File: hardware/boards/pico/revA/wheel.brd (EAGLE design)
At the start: 38 x 38 mm, 0 parts

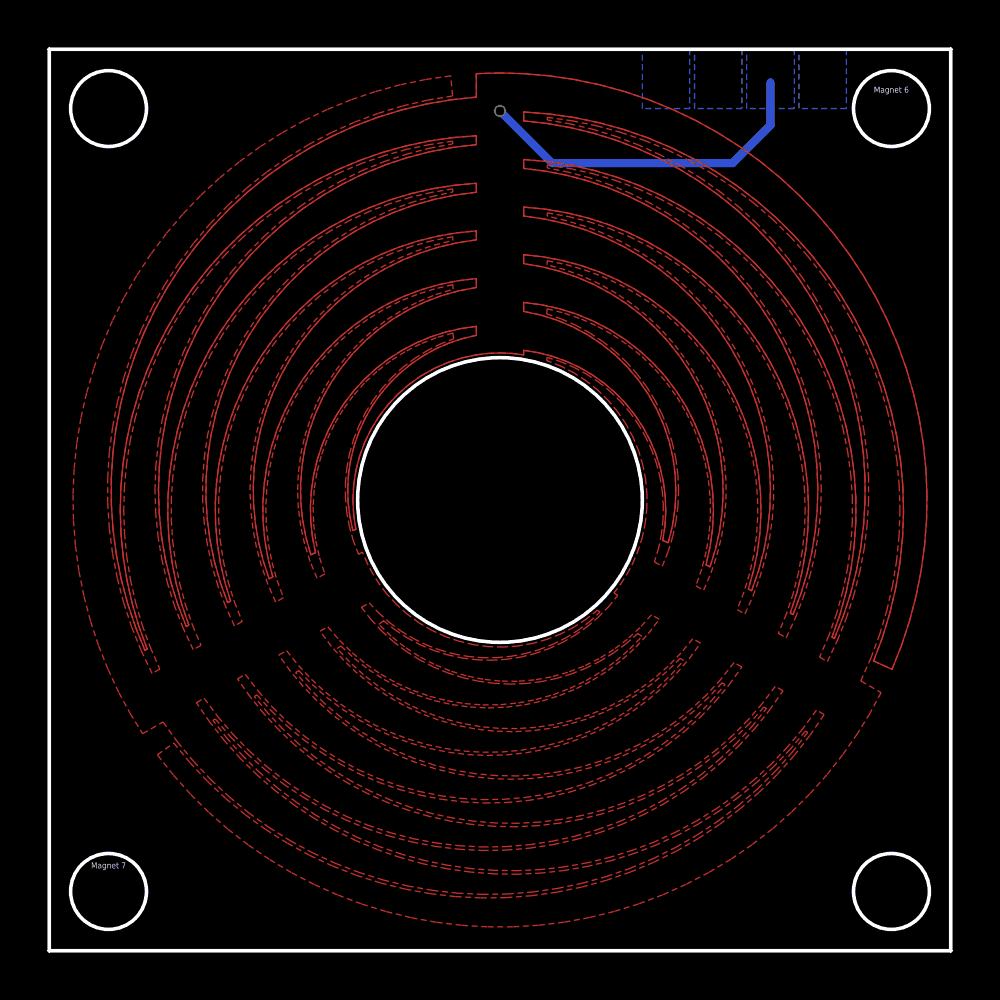
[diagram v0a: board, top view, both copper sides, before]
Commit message: pico: wheel board, basically complete
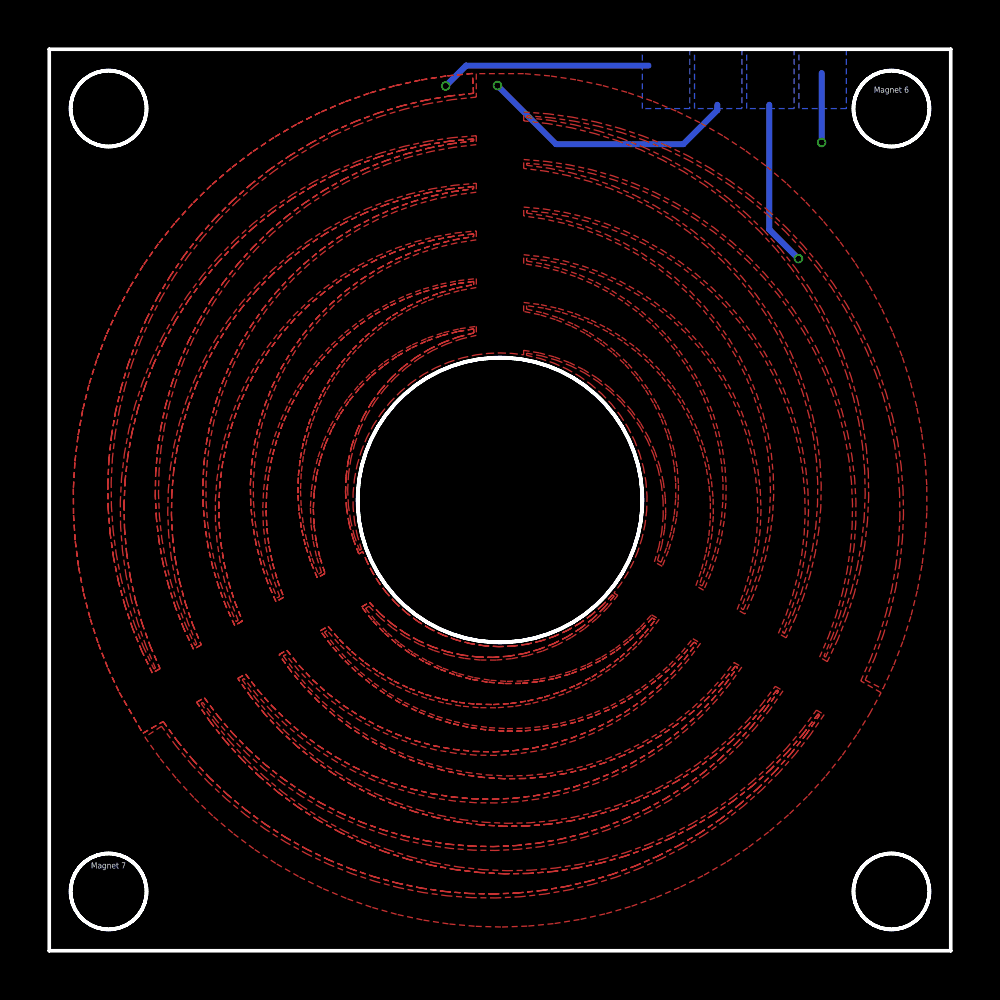
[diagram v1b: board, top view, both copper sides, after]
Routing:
- net CH2: track 473.8 -> 7.00 mm
- net CH1: track 0.00 -> 11.1 mm, vias 0 -> 1
- net CH0: track 0.00 -> 8.91 mm, vias 0 -> 1
- net GUARD: track 0.00 -> 2.93 mm, vias 0 -> 1
- added copper zone on layer 1, net CH3
- added copper zone on layer 1, net GUARD
